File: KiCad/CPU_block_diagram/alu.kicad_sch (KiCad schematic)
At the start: 8 parts, among them U16 74LS245, U17 74LS283, U18 74LS283, U19 74LS86, U20 74LS86, U21 74LS02, U22 74LS08

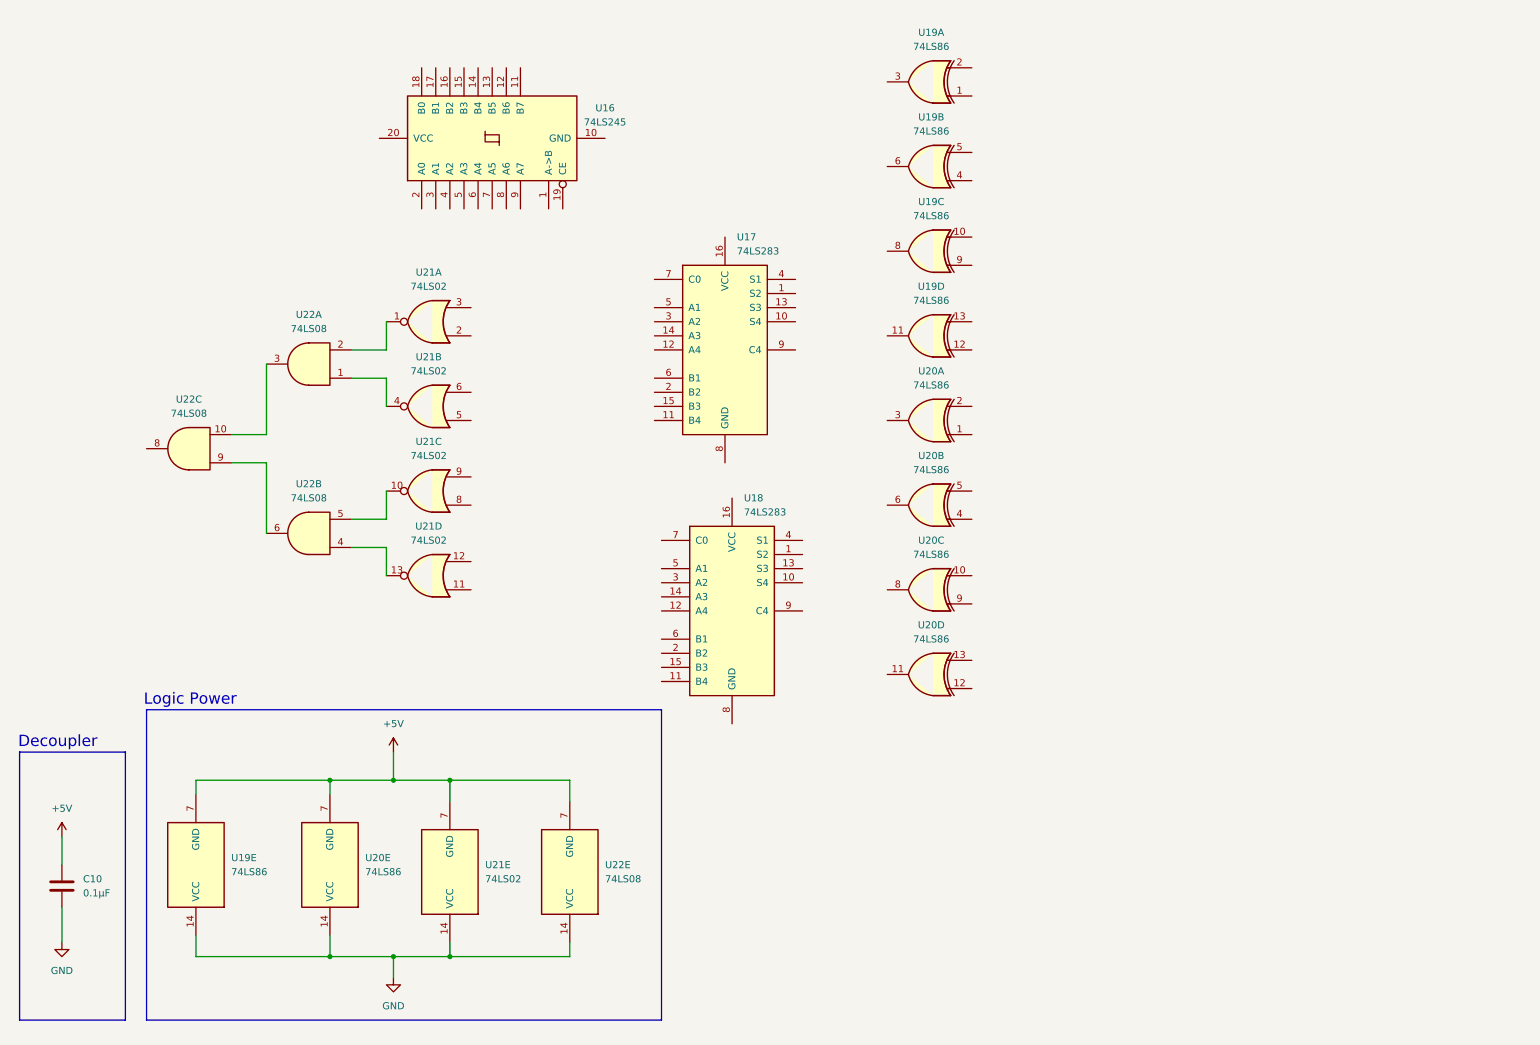
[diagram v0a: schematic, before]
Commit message: vault backup: 2026-01-15 04:46:33
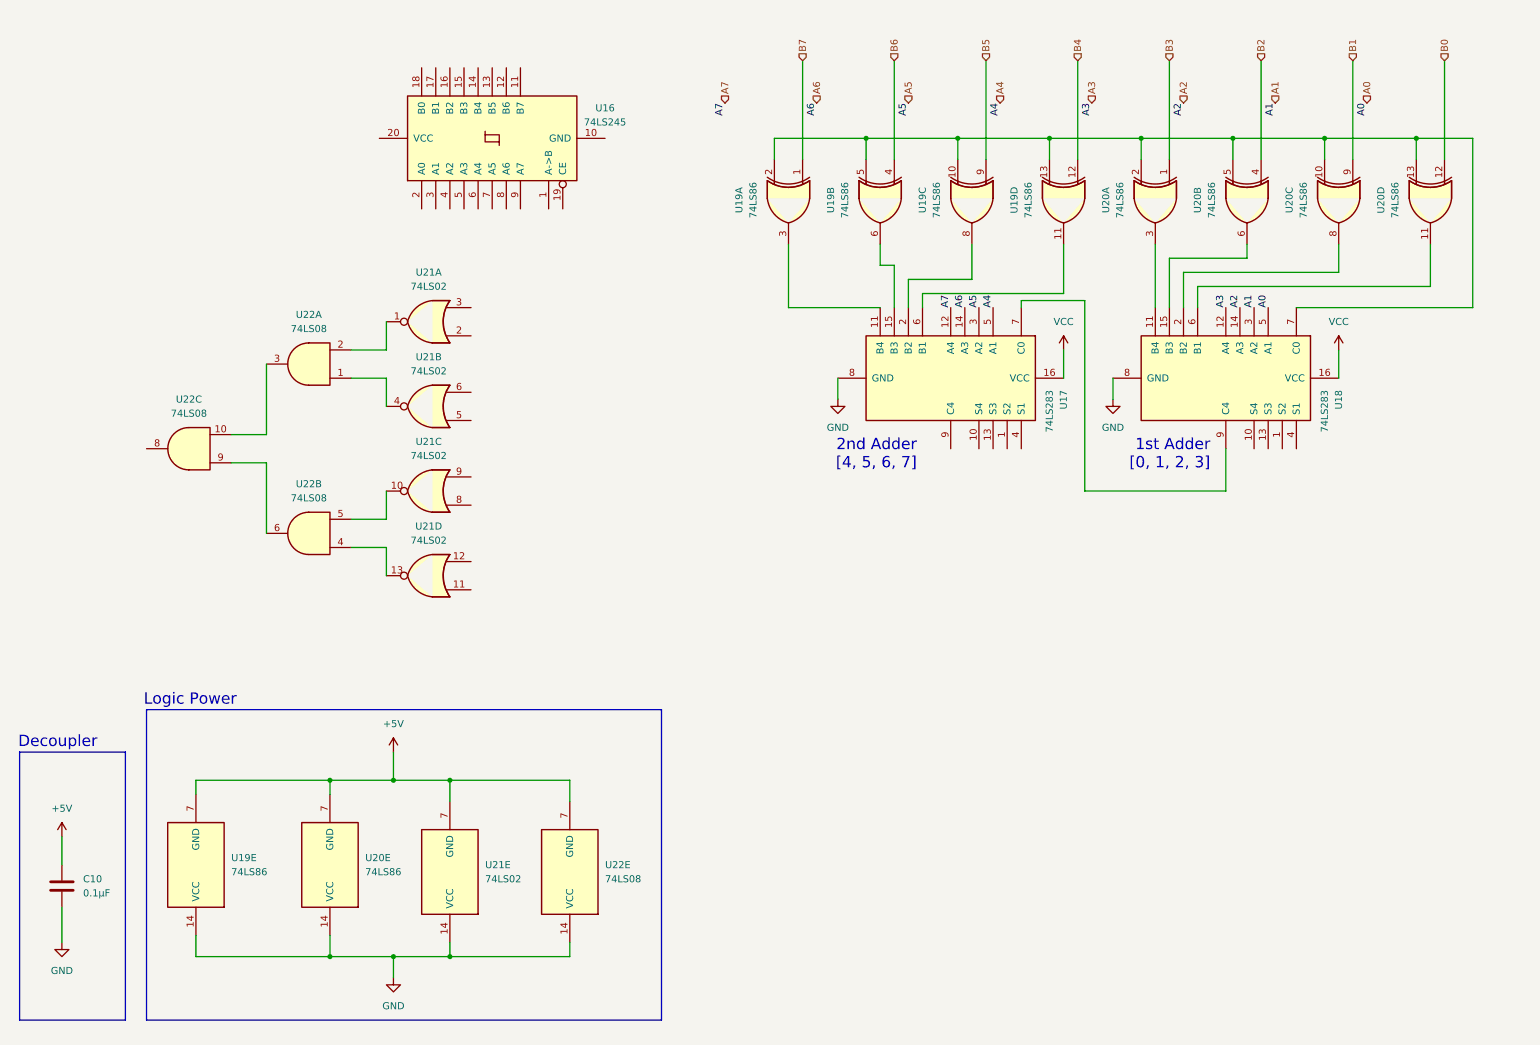
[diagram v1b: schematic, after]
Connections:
- net GND: now also U17.8 (GND), U18.8 (GND)
- net B2: now reaches U20.4
- net at U20.5: now also U18.7 (C0), U19.10, U19.13, U19.2, U19.5, U20.10, U20.13, U20.2
- net at U20.6: now also U18.15 (B3)
- net at U19.11: now also U17.6 (B1)
- net B4: now reaches U19.12
- net at U17.11 (B4): now also U19.3
- net A7: now reaches U17.12 (A4)
- net A6: now reaches U17.14 (A3)
- net at U17.15 (B3): now also U19.6
- net VCC: now reaches U17.16 (VCC)
- net VCC: now also U18.16 (VCC)
- net at U17.2 (B2): now also U19.8
- net A5: now reaches U17.3 (A2)
- net A4: now reaches U17.5 (A1)
- net at U17.7 (C0): now also U18.9 (C4)
- net at U18.11 (B4): now also U20.3
- net A3: now reaches U18.12 (A4)
- net A2: now reaches U18.14 (A3)
- net at U18.2 (B2): now also U20.8
- net A1: now reaches U18.3 (A2)
- net A0: now reaches U18.5 (A1)
- net at U18.6 (B1): now also U20.11
- net B1: now reaches U20.9
- net B0: now reaches U20.12
- net B5: now reaches U19.9
- net B6: now reaches U19.4
- net B7: now reaches U19.1
- net B3: now reaches U20.1
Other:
- note added: "1st Adder [0, 1, 2, 3]"
- note added: "2nd Adder [4, 5, 6, 7]"
- moved on the sheet: U17, U18, U19A, U19B, U19C, U19D, U20A, U20B, U20C, U20D

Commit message: vault backup: 2026-01-15 14:00:21
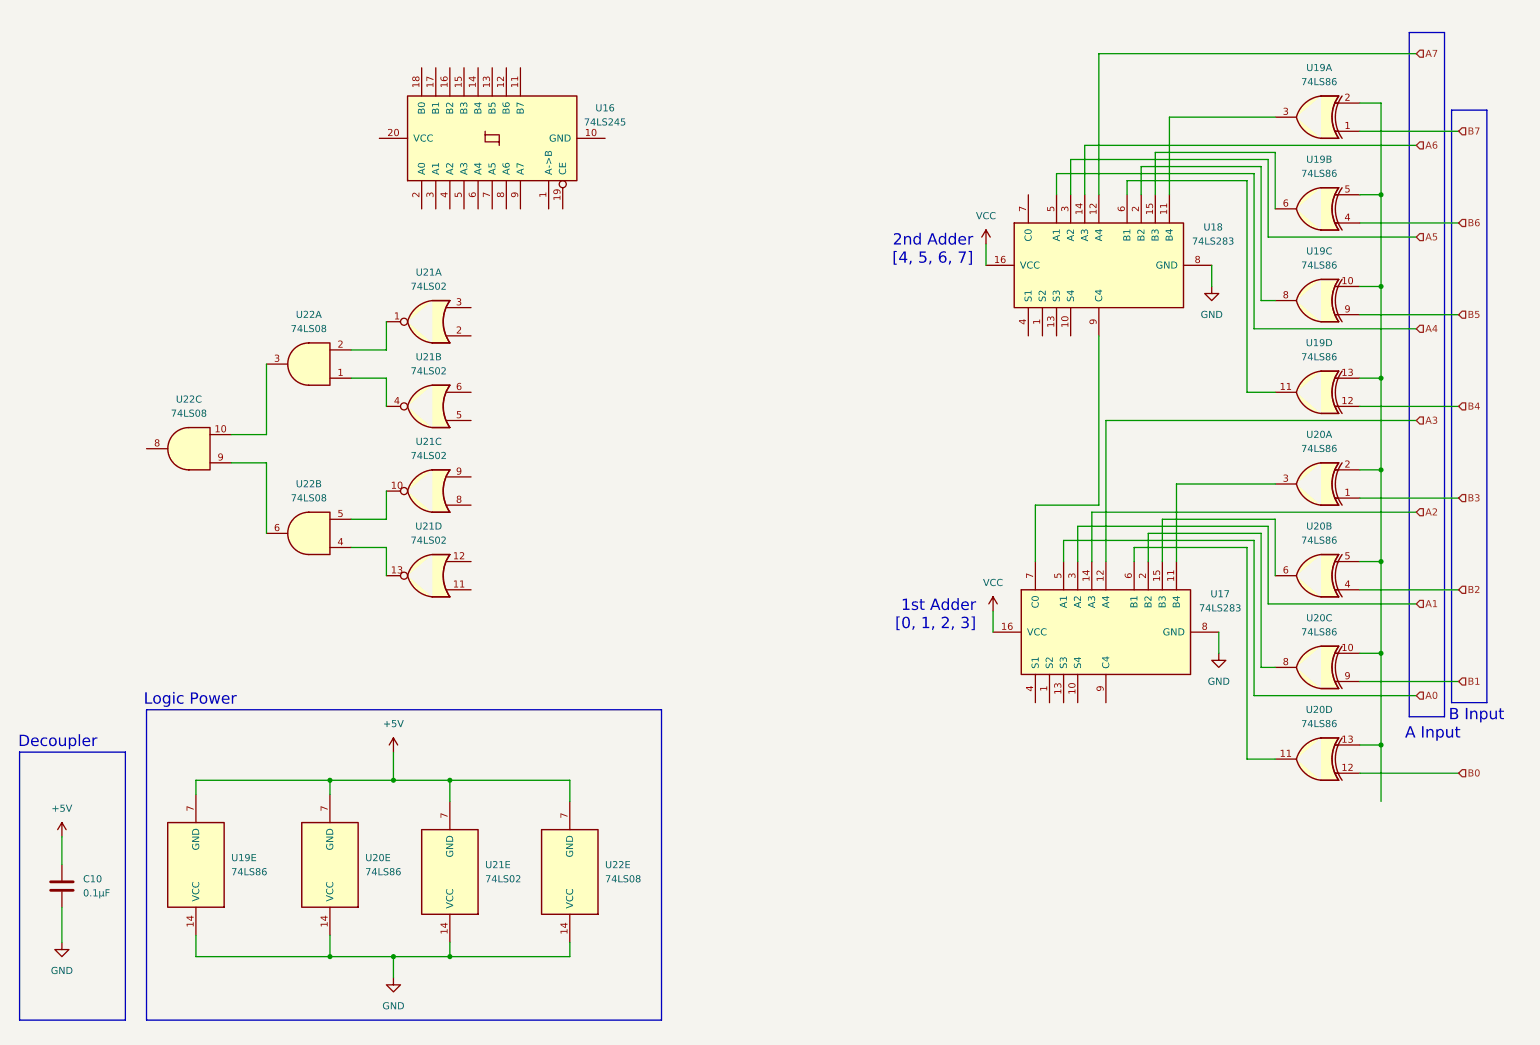
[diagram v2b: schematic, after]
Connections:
- net A0: now also U17.5 (A1); no longer U18.5 (A1)
- net A1: now also U17.3 (A2); no longer U18.3 (A2)
- net A2: now also U17.14 (A3); no longer U18.14 (A3)
- net A3: now also U17.12 (A4); no longer U18.12 (A4)
- net A4: now also U18.5 (A1); no longer U17.5 (A1)
- net A5: now also U18.3 (A2); no longer U17.3 (A2)
- net A6: now also U18.14 (A3); no longer U17.14 (A3)
- net A7: now also U18.12 (A4); no longer U17.12 (A4)
- net at U19.10, U19.13, U19.2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: no longer U18.7 (C0)
- net at U18.15 (B3): now also U19.6; no longer U20.6
- net at U19.11: now also U18.6 (B1); no longer U17.6 (B1)
- net at U19.3: now also U18.11 (B4); no longer U17.11 (B4)
- net at U17.15 (B3): now also U20.6; no longer U19.6
- net at U19.8: now also U18.2 (B2); no longer U17.2 (B2)
- net at U20.3: now also U17.11 (B4); no longer U18.11 (B4)
- net at U20.8: now also U17.2 (B2); no longer U18.2 (B2)
- net at U20.11: now also U17.6 (B1); no longer U18.6 (B1)
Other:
- note added: "A Input"
- note added: "B Input"
- moved on the sheet: U19A, U19B, U19C, U19D, U20A, U20B, U20C, U20D

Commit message: vault backup: 2026-01-16 02:22:53
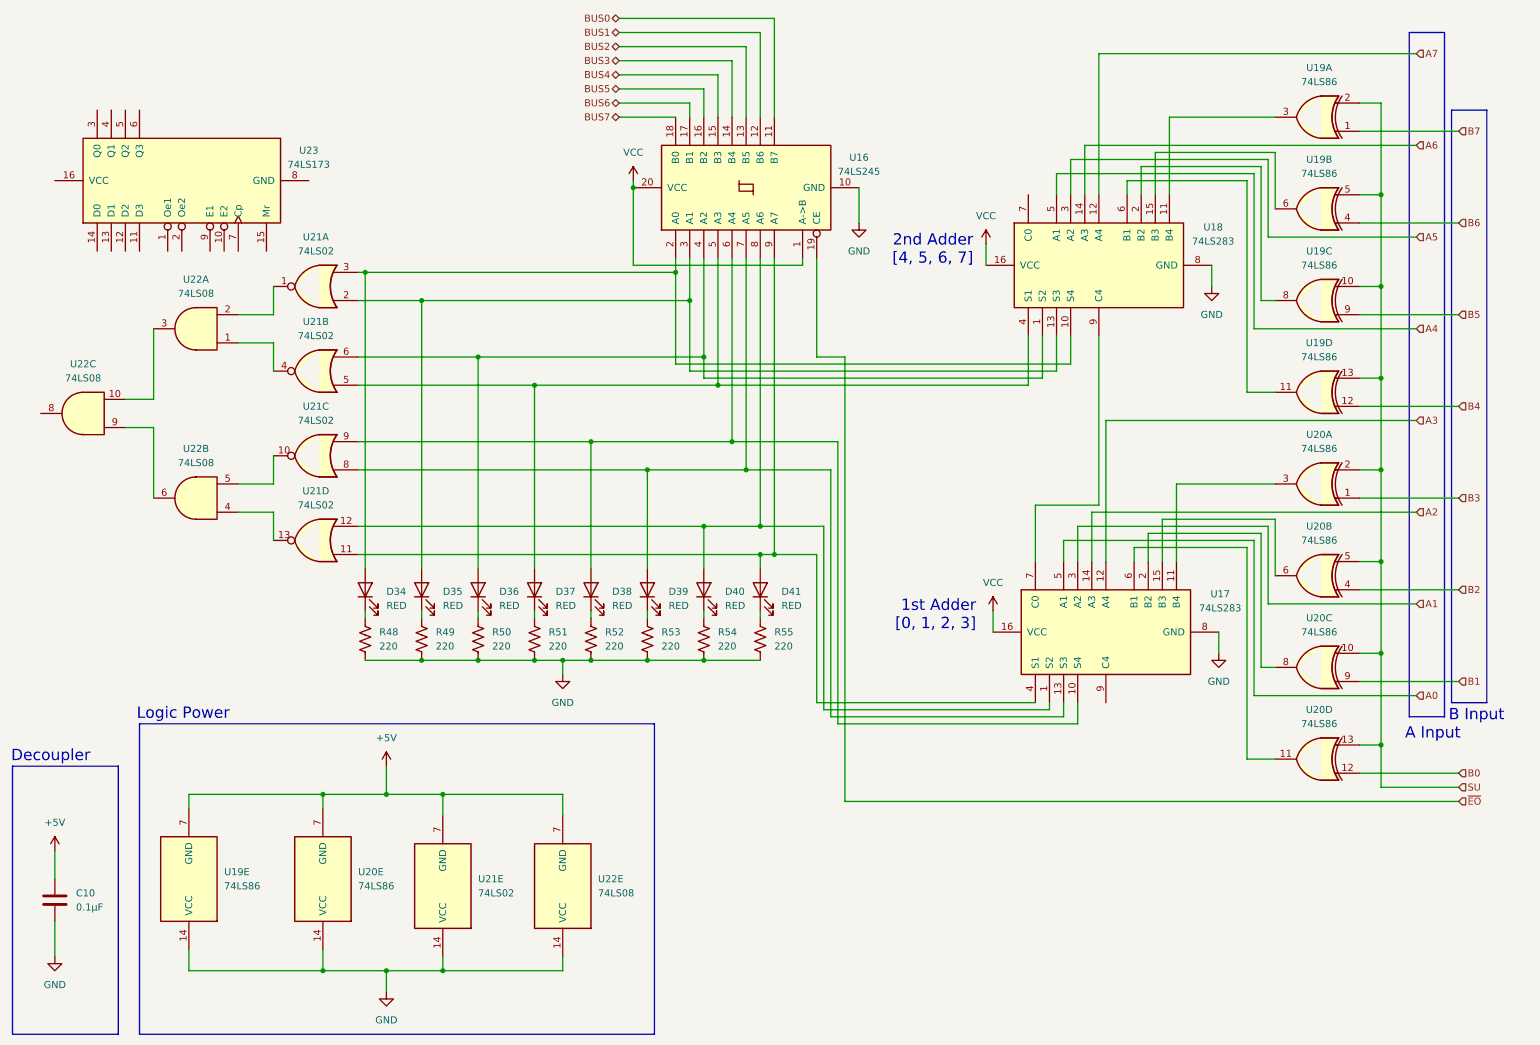
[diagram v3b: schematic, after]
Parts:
- added D34, D35, D36, D37, D38, D39, D40, D41: RED, symbol Device:LED
- added R48, R49, R50, R51, R52, R53, R54, R55: 220, symbol Device:R_US
- added U23: 74LS173, symbol 74xx:74LS173
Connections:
- net GND: now also U16.10 (GND), R48.2, R49.2, R50.2, R51.2, R52.2, R53.2, R54.2, R55.2
- net VCC: now also U16.1 (A->B), U16.20 (VCC)
- net at U18.1 (S2): now also U16.4 (A2), U21.6, D36.2 (A)
- net at U18.10 (S4): now also U16.2 (A0), U21.3, D34.2 (A)
- net at U18.13 (S3): now also U16.3 (A1), U21.2, D35.2 (A)
- net at U18.4 (S1): now also U16.5 (A3), U21.5, D37.2 (A)
- net at U17.1 (S2): now also U16.8 (A6), U21.12, D40.2 (A)
- net at U17.10 (S4): now also U16.6 (A4), U21.9, D38.2 (A)
- net at U17.13 (S3): now also U16.7 (A5), U21.8, D39.2 (A)
- net at U17.4 (S1): now also U16.9 (A7), U21.11, D41.2 (A)
- net SU: now reaches U19.10, U19.13, U19.2, U19.5, U20.10, U20.13, U20.2, U20.5
- net BUS0: now reaches U16.11 (B7)
- net BUS1: now reaches U16.12 (B6)
- net BUS2: now reaches U16.13 (B5)
- net BUS3: now reaches U16.14 (B4)
- net BUS4: now reaches U16.15 (B3)
- net BUS5: now reaches U16.16 (B2)
- net BUS6: now reaches U16.17 (B1)
- net BUS7: now reaches U16.18 (B0)
- net ~{EO}: now reaches U16.19 (CE)
- new net: D38.1 (K), R52.1
- new net: D40.1 (K), R54.1
- new net: D41.1 (K), R55.1
- new net: D39.1 (K), R53.1
- new net: D36.1 (K), R50.1
- new net: D35.1 (K), R49.1
- new net: D37.1 (K), R51.1
- new net: D34.1 (K), R48.1
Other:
- moved on the sheet: C10, U16, U19E, U20E, U21A, U21B, U21C, U21D, U21E, U22A, U22B, U22C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
